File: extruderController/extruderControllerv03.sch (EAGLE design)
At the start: 73 parts, among them IC1 LM1117MPX-5.0, IC2 MAX3467CPA, IC3 ATMEGA2561-16AU, IC4 ULN2003AD, J1 RJ45, Q2 PH7030L, Q3 PH7030L, Q4 PH7030L, Q5 PH7030L, Q6 PH7030L, X1 22-23-2081, X2 22-23-2081, X3 22-23-2101, X6 22-23-2041, X8 22-23-2031, X9 22-23-2031

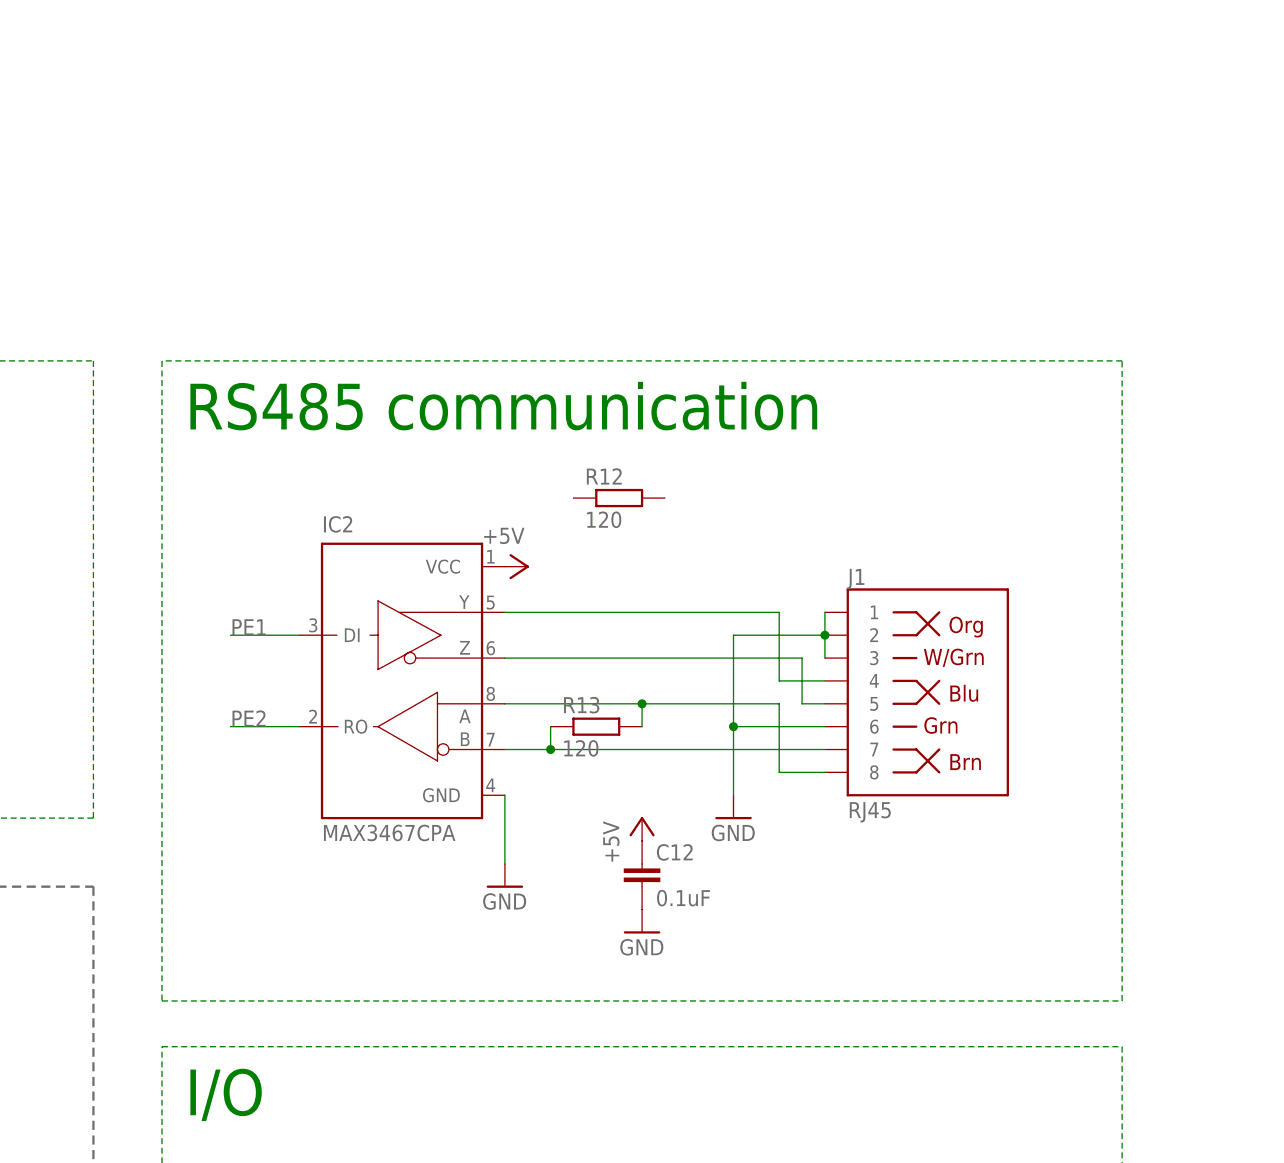
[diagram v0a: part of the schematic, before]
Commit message: f
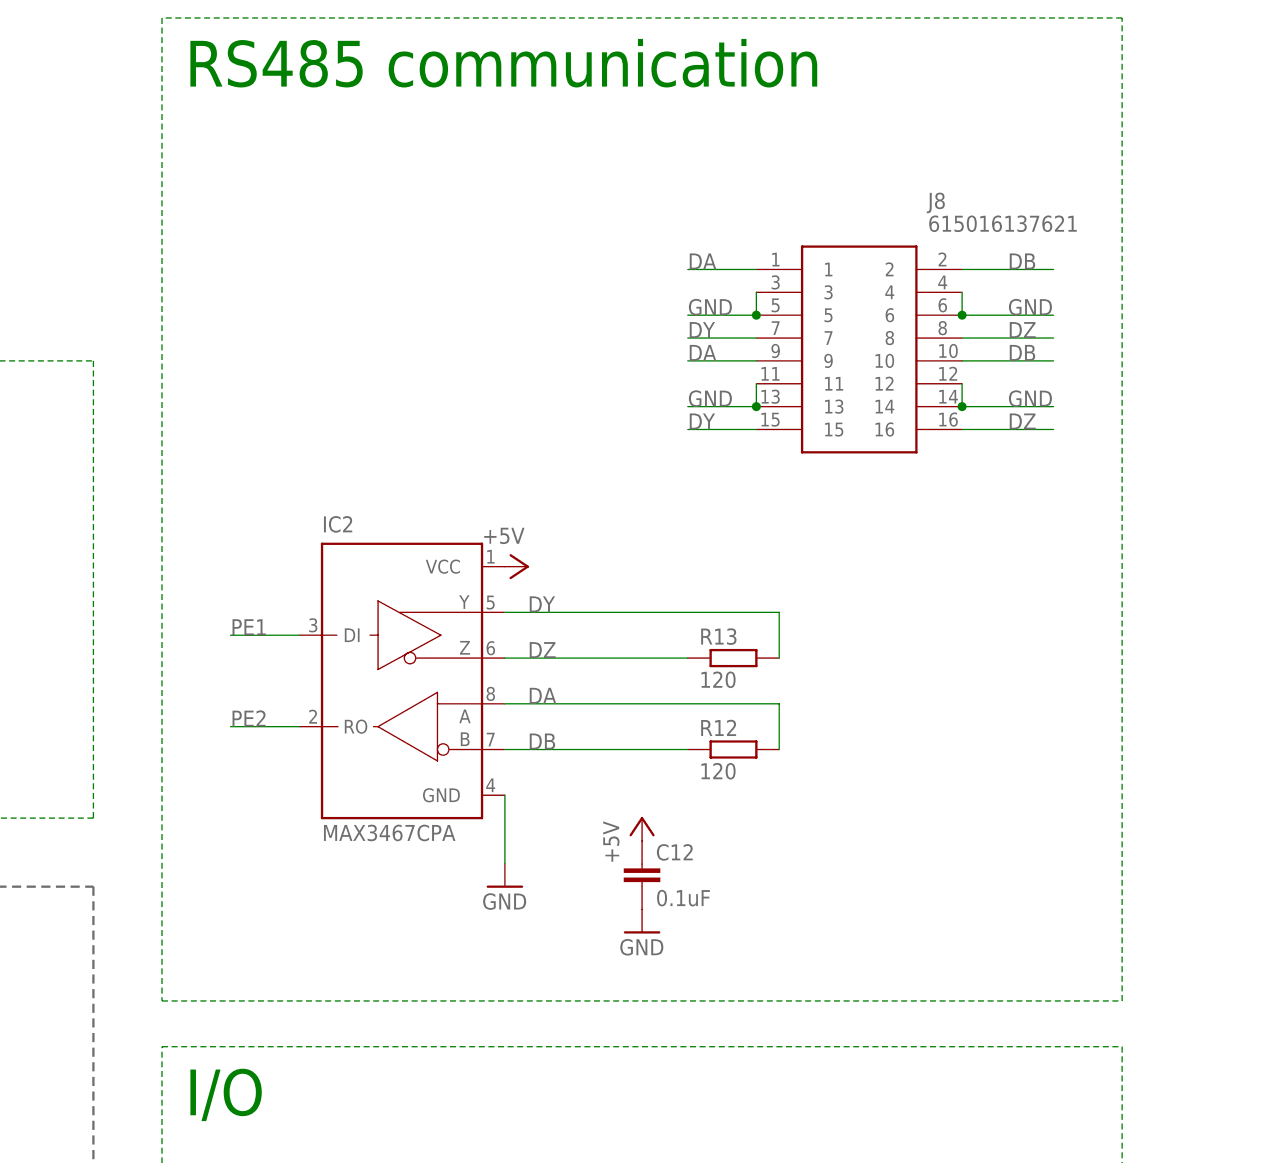
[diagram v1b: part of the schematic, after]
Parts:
- removed J1: RJ45, SparkFun-Connectors:RJ45-8
- added J8: 615016137621, SamacSys_Parts:615016137621
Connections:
- removed net N$27: IC2.B, J1.7, R13.1
- removed net N$35: IC2.Y, J1.4
- removed net N$36: IC2.A, J1.8, R13.2
- removed net N$45: IC2.Z, J1.5
- new net DA: IC2.A, J8.1, J8.9, R12.2
- new net DB: IC2.B, J8.10, J8.2, R12.1
- new net DY: IC2.Y, J8.15, J8.7, R13.2
- new net DZ: IC2.Z, J8.16, J8.8, R13.1
- net GND: now also J8.11, J8.12, J8.13, J8.14, J8.3, J8.4, J8.5, J8.6; no longer J1.1, J1.2, J1.3, J1.6
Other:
- moved on the sheet: R12, R13

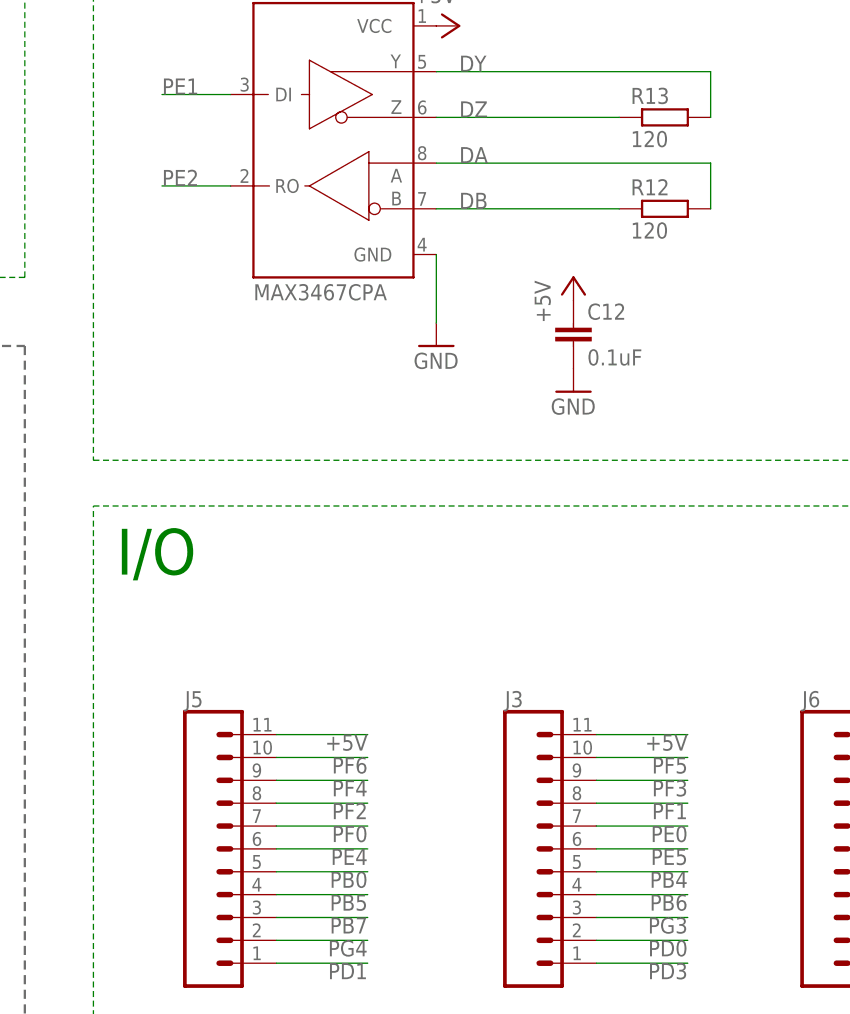
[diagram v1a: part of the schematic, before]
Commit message: e
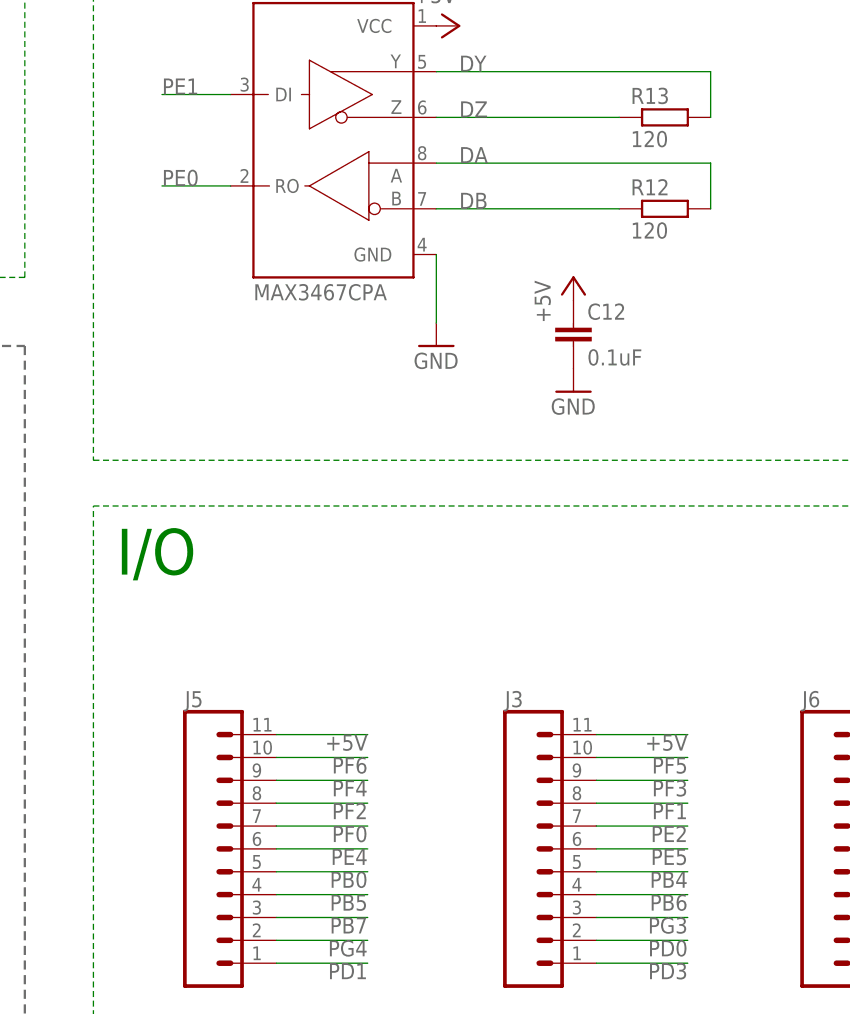
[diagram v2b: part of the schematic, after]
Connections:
- net PE0: now also IC2.RO; no longer J3.7
- net PE2: now also J3.7; no longer IC2.RO
